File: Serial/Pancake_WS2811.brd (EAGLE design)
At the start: 14.2 x 10.7 mm, 14 parts

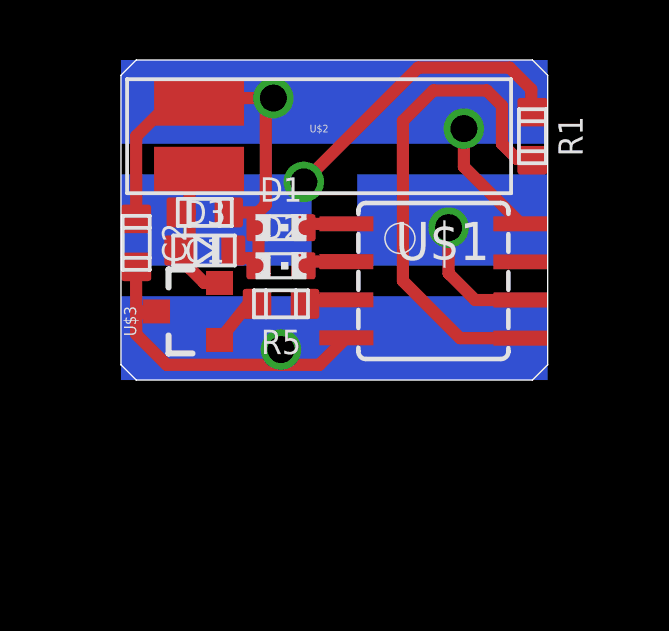
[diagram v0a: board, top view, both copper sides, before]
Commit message: Update pictures, pancake
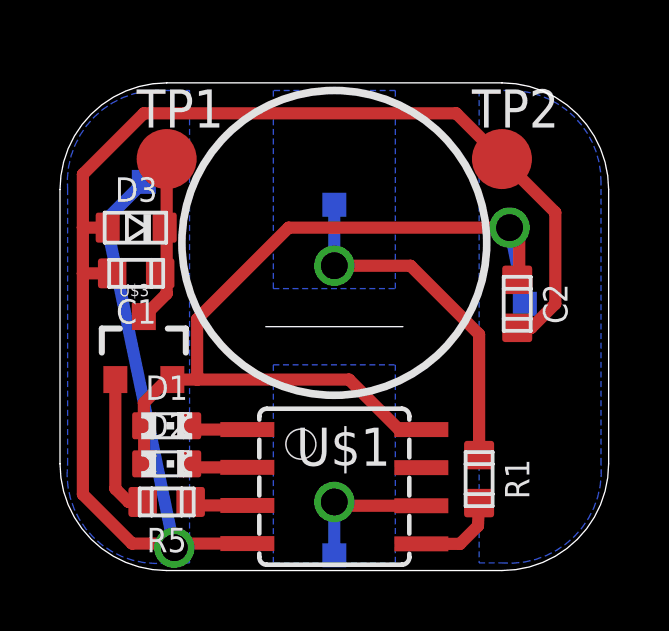
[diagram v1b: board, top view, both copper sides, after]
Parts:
- removed U$2: PINHD_2VIBRATIONSMOTO_303-103, thar:VIBRATIONSMOTOR303-103
- added TP1, TP2: TPTP20R, testpad:TP20R
- moved C2 12.9 mm to (29.7, 28.4)
- moved R1 11.6 mm to (28.4, 22.6)
- moved DI 11.1 mm to (23.6, 20.1)
- moved VCC 9.35 mm to (30.0, 28.4)
- moved D1 7.62 mm to (18.0, 24.4)
- moved D2 7.62 mm to (18.0, 23.1)
- moved R5 7.62 mm to (18.0, 21.8)
- moved U$1 7.61 mm to (23.6, 22.4)
- moved GND 7.12 mm to (17.3, 32.5)
- moved C1 3.06 mm to (17.0, 29.5)
- moved D3 2.41 mm to (17.0, 31.0)
- moved U$3 1.98 mm to (17.3, 26.9), turned to 0 degrees
- moved DO 1.37 mm to (23.6, 31.8)
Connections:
- removed net N$4: C1.1, D3.A, U$2.2, U$3.2
- new net N$1: C1.2, D3.C, TP1.TP, U$3.3
- net GND: now also C1.1, D3.A, TP2.TP; no longer U$3.3
- net VCC: now also U$3.2; no longer C1.2, D3.C, U$2.1
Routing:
- net GND: track 12.5 -> 54.5 mm
- net N$2: track 16.9 -> 2.90 mm
- net N$1: track 0.00 -> 5.94 mm
- net N$4: track 5.52 -> 0.00 mm
- net VCC: track 27.2 -> 30.5 mm, vias 2 -> 1
- net N$10: track 1.85 -> 4.73 mm
- net N$3: track 10.8 -> 11.9 mm
- net N$7: track 1.56 -> 2.07 mm
- added copper zone on layer 16, net DIN
- added copper zone on layer 16, net GND
- added copper zone on layer 16, net N$3
- added copper zone on layer 16, net VCC
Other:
- board size 14.2 x 10.7 mm -> 18.3 x 16.3 mm
